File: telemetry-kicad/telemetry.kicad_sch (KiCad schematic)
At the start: 98 parts, among them J1 2601-1102, J2 RFPC-SMA27-F, J3 TC2030, J4 2601-1102, J5 2601-1102, J6 USB_C_Receptacle_USB2.0_16P, J7 SD_Card_Receptacle, Q1 DMP3099LQ-7, SW1 SW_NRST, SW2 SW_BOOT0, U1 LMR33610ADDAR, U10 TLC59108IPWR, U11 MCP1703T-5002E/CB, U2 ASM330LHHXG1TR, U3 MAX-M10S-00B, U4 TCAN337, U5 STM32H523RCT7, U6 TCAN337, U7 USBLC6-2SC6, U9 TLC59108IPWR, Y1 ABM8AIG-24.000MHz-8-2Z-T

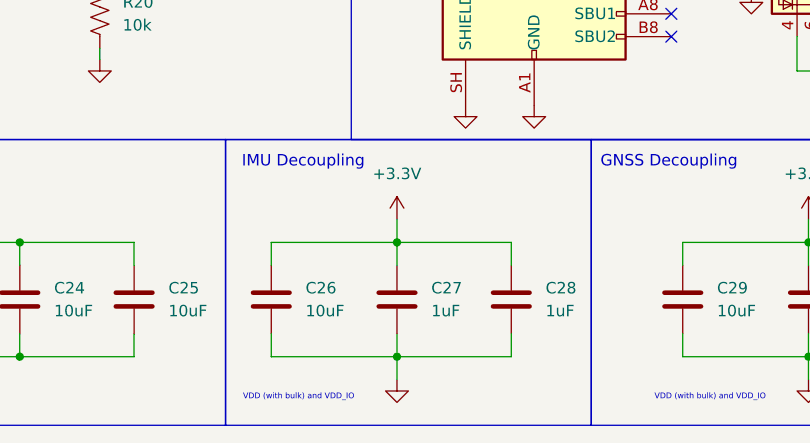
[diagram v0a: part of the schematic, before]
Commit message: PCB draft complete
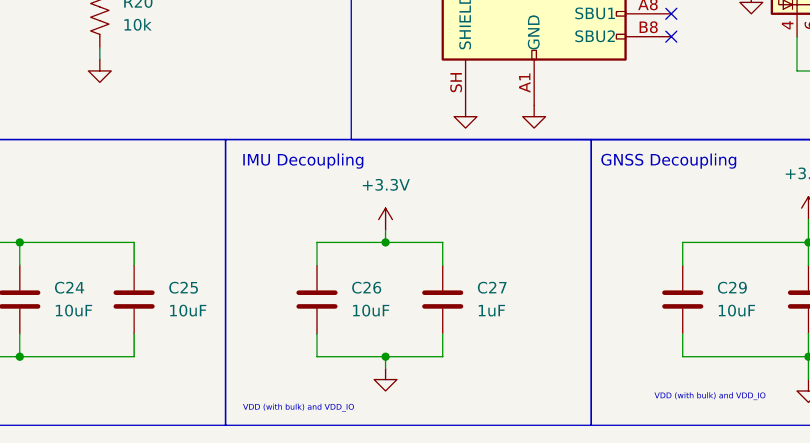
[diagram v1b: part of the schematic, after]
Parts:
- removed C28: 1uF, Capacitor_SMD:C_0805_2012Metric_Pad1.18x1.45mm_HandSolder, symbol Device:C
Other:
- moved on the sheet: C26, C27
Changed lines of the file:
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@@
 	(text "VDD (with bulk) and VDD_IO"
 		(exclude_from_sim no)
-		(at 130.048 257.302 0)
+		(at 130.048 258.572 0)
 		(effects
 			(font
@@
 	)
 	(junction
+		(at 139.7 252.73)
+		(diameter 0)
+		(color 0 0 0 0)
+	)
+	(junction
 		(at 57.15 41.91)
 		(diameter 0)
@@
 	)
 	(junction
-		(at 186.69 252.73)
+		(at 139.7 240.03)
 		(diameter 0)
 		(color 0 0 0 0)
 	)
 	(junction
-		(at 422.91 113.03)
+		(at 186.69 252.73)
 		(diameter 0)
 		(color 0 0 0 0)
 	)
 	(junction
-		(at 232.41 237.49)
+		(at 422.91 113.03)
 		(diameter 0)
 		(color 0 0 0 0)
 	)
 	(junction
-		(at 93.98 31.75)
+		(at 232.41 237.49)
 		(diameter 0)
 		(color 0 0 0 0)
 	)
 	(junction
-		(at 140.97 240.03)
+		(at 93.98 31.75)
 		(diameter 0)
 		(color 0 0 0 0)
@@
 	)
 	(junction
-		(at 140.97 252.73)
-		(diameter 0)
-		(color 0 0 0 0)
-	)
-	(junction
 		(at 186.69 240.03)
 		(diameter 0)
@@
 	(wire
 		(pts
-			(xy 153.67 240.03) (xy 153.67 242.57)
-		)
-		(stroke
-			(width 0)
-			(type default)
-		)
-	)
-	(wire
-		(pts
 			(xy 172.72 124.46) (xy 172.72 119.38)
 		)
@@
 	(wire
 		(pts
-			(xy 140.97 237.49) (xy 140.97 240.03)
+			(xy 139.7 238.76) (xy 139.7 240.03)
 		)
 		(stroke
@@
 	(wire
 		(pts
-			(xy 140.97 250.19) (xy 140.97 252.73)
+			(xy 146.05 250.19) (xy 146.05 252.73)
 		)
 		(stroke
@@
 	(wire
 		(pts
-			(xy 140.97 240.03) (xy 140.97 242.57)
-		)
-		(stroke
-			(width 0)
-			(type default)
-		)
-	)
-	(wire
-		(pts
-			(xy 153.67 252.73) (xy 153.67 250.19)
+			(xy 146.05 240.03) (xy 146.05 242.57)
 		)
 		(stroke
@@
 	(wire
 		(pts
-			(xy 140.97 240.03) (xy 153.67 240.03)
-		)
-		(stroke
-			(width 0)
-			(type default)
-		)
-	)
-	(wire
-		(pts
 			(xy 194.31 172.72) (xy 195.58 172.72)
 		)
@@
 	(wire
 		(pts
-			(xy 127 240.03) (xy 140.97 240.03)
+			(xy 132.08 240.03) (xy 139.7 240.03)
 		)
 		(stroke
@@
 	(wire
 		(pts
-			(xy 127 250.19) (xy 127 252.73)
+			(xy 132.08 250.19) (xy 132.08 252.73)
 		)
 		(stroke
@@
 	(wire
 		(pts
-			(xy 127 242.57) (xy 127 240.03)
+			(xy 132.08 242.57) (xy 132.08 240.03)
 		)
 		(stroke
@@
 	(wire
 		(pts
-			(xy 140.97 252.73) (xy 153.67 252.73)
-		)
-		(stroke
-			(width 0)
-			(type default)
-		)
-	)
-	(wire
-		(pts
 			(xy 124.46 114.3) (xy 123.19 114.3)
 		)
@@
 	(wire
 		(pts
+			(xy 139.7 240.03) (xy 146.05 240.03)
+		)
+		(stroke
+			(width 0)
+			(type default)
+		)
+	)
+	(wire
+		(pts
+			(xy 139.7 252.73) (xy 146.05 252.73)
+		)
+		(stroke
+			(width 0)
+			(type default)
+		)
+	)
+	(wire
+		(pts
 			(xy 238.76 39.37) (xy 238.76 34.29)
 		)
@@
 	(wire
 		(pts
-			(xy 127 252.73) (xy 140.97 252.73)
+			(xy 132.08 252.73) (xy 139.7 252.73)
 		)
 		(stroke
@@
 	(wire
 		(pts
-			(xy 140.97 252.73) (xy 140.97 255.27)
+			(xy 139.7 252.73) (xy 139.7 254)
 		)
 		(stroke
@@
 	(symbol
 		(lib_id "Device:C")
-		(at 140.97 246.38 0)
+		(at 146.05 246.38 0)
 		(unit 1)
 		(body_style 1)
@@
 		(fields_autoplaced yes)
 		(property "Reference" "C27"
-			(at 144.78 245.1099 0)
+			(at 149.86 245.1099 0)
 			(show_name no)
 			(do_not_autoplace no)
@@
 		)
 		(property "Value" "1uF"
-			(at 144.78 247.6499 0)
+			(at 149.86 247.6499 0)
 			(show_name no)
 			(do_not_autoplace no)
@@
 		)
 		(property "Footprint" "Capacitor_SMD:C_0805_2012Metric_Pad1.18x1.45mm_HandSolder"
-			(at 141.9352 250.19 0)
+			(at 147.0152 250.19 0)
 			(hide yes)
 			(show_name no)
@@
 		)
 		(property "Datasheet" ""
-			(at 140.97 246.38 0)
+			(at 146.05 246.38 0)
 			(hide yes)
 			(show_name no)
@@
 		)
 		(property "Description" "Unpolarized capacitor"
-			(at 140.97 246.38 0)
+			(at 146.05 246.38 0)
 			(hide yes)
 			(show_name no)
@@
 	(symbol
 		(lib_id "power:+3.3V")
-		(at 140.97 237.49 0)
+		(at 139.7 238.76 0)
 		(unit 1)
 		(body_style 1)
@@
 		(fields_autoplaced yes)
 		(property "Reference" "#PWR076"
-			(at 140.97 241.3 0)
+			(at 139.7 242.57 0)
 			(hide yes)
 			(show_name no)
@@
 		)
 		(property "Value" "+3.3V"
-			(at 140.97 232.41 0)
+			(at 139.7 233.68 0)
 			(show_name no)
 			(do_not_autoplace no)
@@
 		)
 		(property "Footprint" ""
-			(at 140.97 237.49 0)
+			(at 139.7 238.76 0)
 			(hide yes)
 			(show_name no)
@@
 		)
 		(property "Datasheet" ""
-			(at 140.97 237.49 0)
+			(at 139.7 238.76 0)
 			(hide yes)
 			(show_name no)
@@
 		)
 		(property "Description" "Power symbol creates a global label with name \"+3.3V\""
-			(at 140.97 237.49 0)
+			(at 139.7 238.76 0)
 			(hide yes)
 			(show_name no)
@@
 	(symbol
 		(lib_id "Device:C")
-		(at 127 246.38 180)
+		(at 132.08 246.38 180)
 		(unit 1)
 		(body_style 1)
@@
 		(fields_autoplaced yes)
 		(property "Reference" "C26"
-			(at 130.81 245.1099 0)
+			(at 135.89 245.1099 0)
 			(show_name no)
 			(do_not_autoplace no)
@@
 		)
 		(property "Value" "10uF"
-			(at 130.81 247.6499 0)
+			(at 135.89 247.6499 0)
 			(show_name no)
 			(do_not_autoplace no)
@@
 		)
 		(property "Footprint" "Capacitor_SMD:C_0805_2012Metric_Pad1.18x1.45mm_HandSolder"
-			(at 126.0348 242.57 0)
+			(at 131.1148 242.57 0)
 			(hide yes)
 			(show_name no)
@@
 		)
 		(property "Datasheet" ""
-			(at 127 246.38 0)
+			(at 132.08 246.38 0)
 			(hide yes)
 			(show_name no)
@@
 		)
 		(property "Description" "Unpolarized capacitor"
-			(at 127 246.38 0)
+			(at 132.08 246.38 0)
 			(hide yes)
 			(show_name no)
@@
 	(symbol
 		(lib_id "power:GND")
-		(at 140.97 255.27 0)
+		(at 139.7 254 0)
 		(unit 1)
 		(body_style 1)
@@
 		(fields_autoplaced yes)
 		(property "Reference" "#PWR081"
-			(at 140.97 261.62 0)
+			(at 139.7 260.35 0)
 			(hide yes)
 			(show_name no)
@@
 		)
 		(property "Value" "GND"
-			(at 140.97 260.35 0)
+			(at 139.7 259.08 0)
 			(hide yes)
 			(show_name no)
@@
 		)
 		(property "Footprint" ""
-			(at 140.97 255.27 0)
+			(at 139.7 254 0)
 			(hide yes)
 			(show_name no)
@@
 		)
 		(property "Datasheet" ""
-			(at 140.97 255.27 0)
+			(at 139.7 254 0)
 			(hide yes)
 			(show_name no)
@@
 		)
 		(property "Description" "Power symbol creates a global label with name \"GND\" , ground"
-			(at 140.97 255.27 0)
+			(at 139.7 254 0)
 			(hide yes)
 			(show_name no)
@@
 					(unit 1)
 				)
-			)
-		)
-	)
-	(symbol
-		(lib_id "Device:C")
-		(at 153.67 246.38 0)
-		(unit 1)
-		(body_style 1)
-		(exclude_from_sim no)
-		(in_bom yes)
-		(on_board yes)
-		(in_pos_files yes)
-		(dnp no)
-		(fields_autoplaced yes)
-		(property "Reference" "C28"
-			(at 157.48 245.1099 0)
-			(show_name no)
-			(do_not_autoplace no)
-			(effects
-				(font
-					(size 1.27 1.27)
-				)
-				(justify left)
-			)
-		)
-		(property "Value" "1uF"
-			(at 157.48 247.6499 0)
-			(show_name no)
-			(do_not_autoplace no)
-			(effects
-				(font
-					(size 1.27 1.27)
-				)
-				(justify left)
-			)
-		)
-		(property "Footprint" "Capacitor_SMD:C_0805_2012Metric_Pad1.18x1.45mm_HandSolder"
-			(at 154.6352 250.19 0)
-			(hide yes)
-			(show_name no)
-			(do_not_autoplace no)
-			(effects
-				(font
-					(size 1.27 1.27)
-				)
-			)
-		)
-		(property "Datasheet" ""
-			(at 153.67 246.38 0)
-			(hide yes)
-			(show_name no)
-			(do_not_autoplace no)
-			(effects
-				(font
-					(size 1.27 1.27)
-				)
-			)
-		)
-		(property "Description" "Unpolarized capacitor"
-			(at 153.67 246.38 0)
-			(hide yes)
-			(show_name no)
-			(do_not_autoplace no)
-			(effects
-				(font
-					(size 1.27 1.27)
-				)
-			)
-		)
-		(pin "1"
-		)
-		(pin "2"
-		)
-		(instances
-			(project "telemetry"
-				(path "/3df6834d-aaf5-42e5-8a41-0f444a5b1186"
-					(reference "C28")
-					(unit 1)
-				)
